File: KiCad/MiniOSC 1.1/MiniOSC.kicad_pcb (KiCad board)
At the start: 2 copper layers, 94.1 x 128.5 mm, 58 parts, among them J1 Conn_01x16_Female, J2 Conn_01x16_Male, J3 V_OCT_IN, J4 FM_IN, J5 PULSE_OUT, J6 SAW_OUT, J7 JST_BUS, J8 IDC_BUS, Q1 BC558, Q2 BC548, U1 TL074, U2 40106

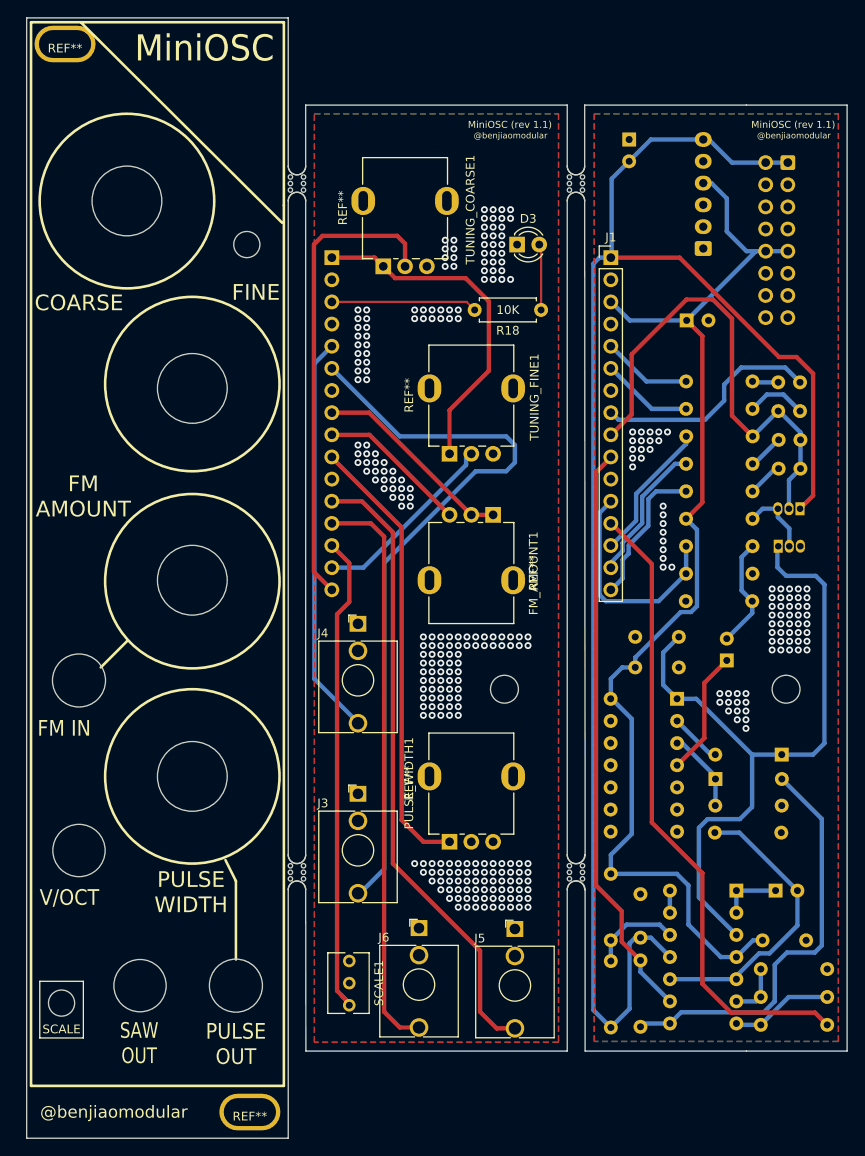
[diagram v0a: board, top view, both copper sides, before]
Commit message: added new branch for v2
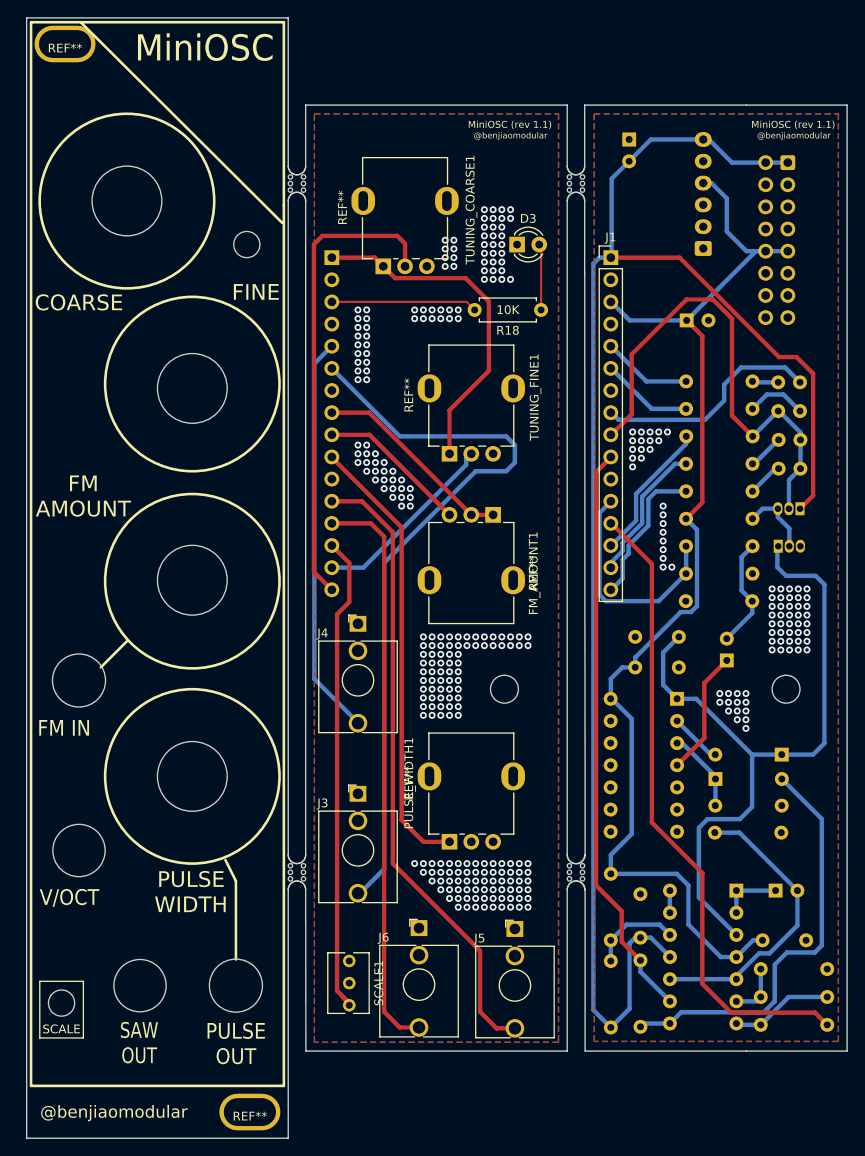
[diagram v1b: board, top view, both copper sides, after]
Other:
- outline, holes or cut-outs redrawn
- net class Default removed
